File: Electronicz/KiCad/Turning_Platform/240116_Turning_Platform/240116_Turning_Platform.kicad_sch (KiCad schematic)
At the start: 11 parts, among them J1 StepperMotor, J2 StepperDriverA, J3 StepperDriverB, J5 +12V, J6 GND, J7 Display, J8 RotaryEncoder

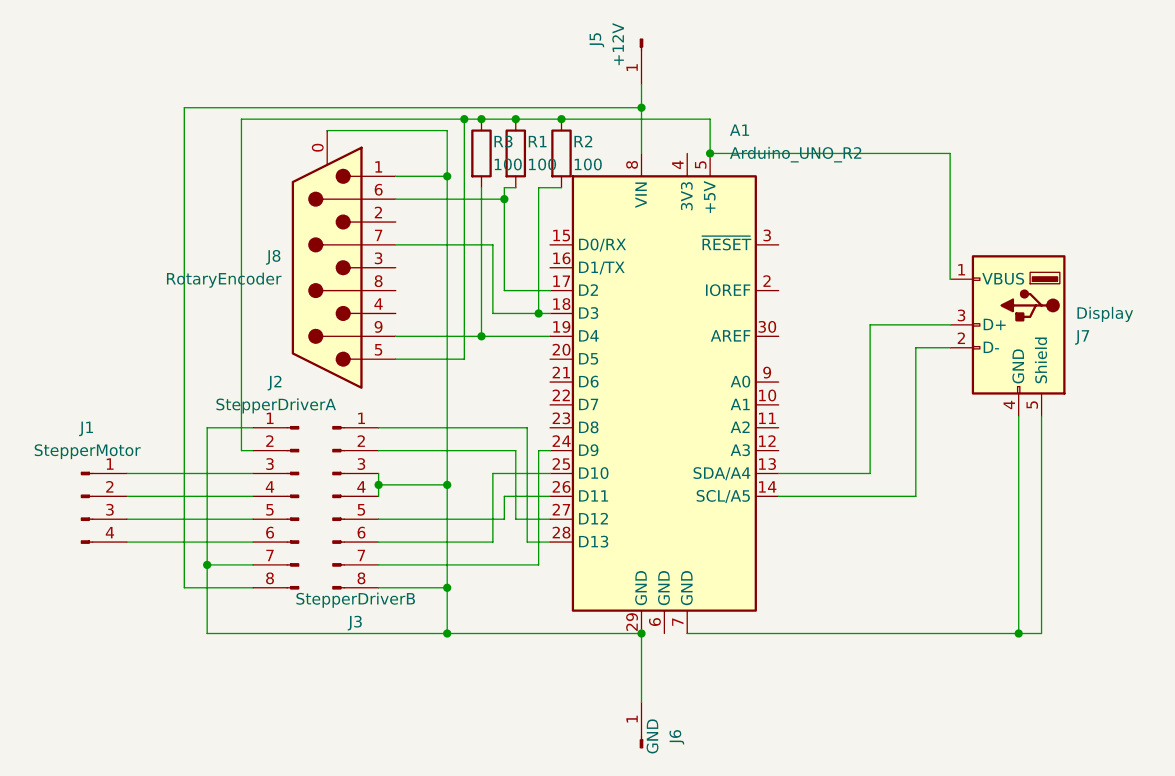
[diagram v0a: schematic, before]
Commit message: Plot Turning Platform PCB
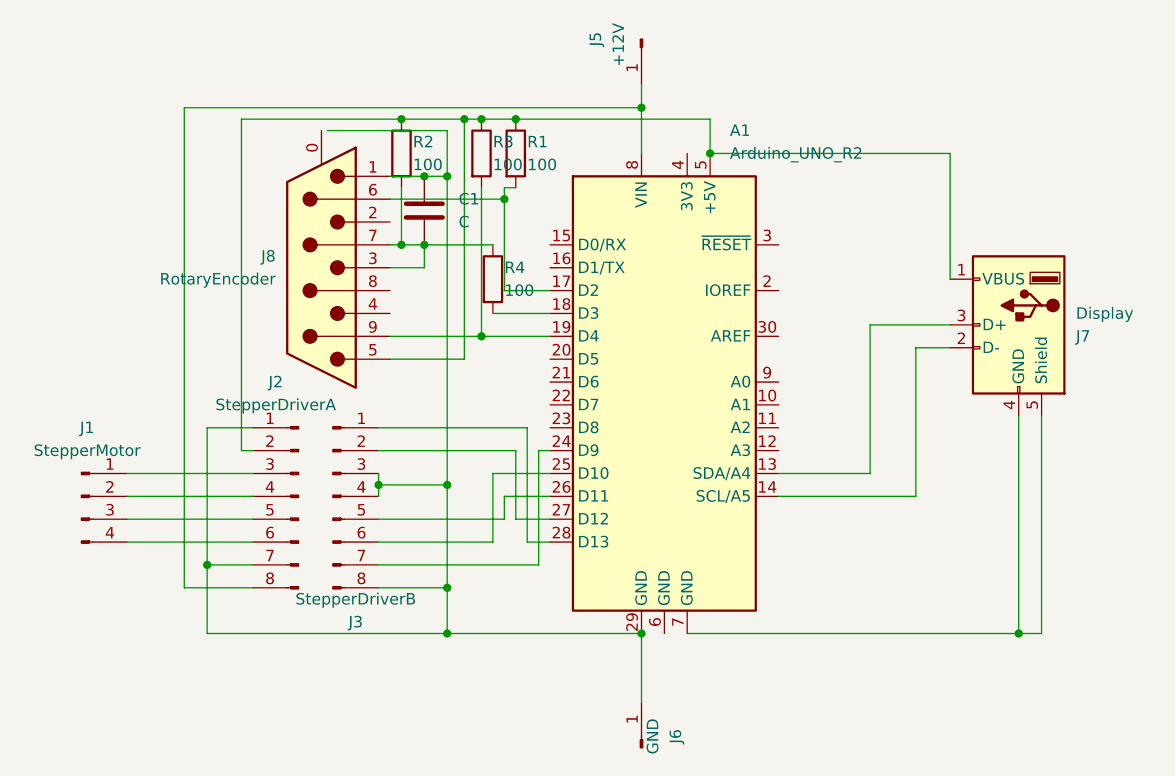
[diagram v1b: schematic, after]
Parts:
- added C1: C, Capacitor_THT:CP_Radial_D10.0mm_P7.50mm, symbol Device:C
- added R4: 100, Resistor_THT:R_Axial_DIN0207_L6.3mm_D2.5mm_P10.16mm_Horizontal, symbol Device:R
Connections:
- net at A1.29 (GND), J2.1 (Pin_1), J2.7 (Pin_7)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: now also C1.1; no longer J8.0 (PAD)
- net at J8.3: now also J8.7, R2.2, C1.2, R4.1
- new net: A1.18 (D3), R4.2
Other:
- moved on the sheet: J8
